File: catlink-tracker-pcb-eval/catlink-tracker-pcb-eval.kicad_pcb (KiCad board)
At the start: 4 copper layers, 36.4 x 38.8 mm, 42 parts, among them J1 S2B-PH-K, J2 U.FL, J3 Header_01x03, J4 Header_02x02, J5 Header_02x03, J6 Header_01x02, J7 Header_01x06, J8 Header_01x05, SW1 SW_Push, U1 STM32L412K8Tx, U2 TLV75530PDBV, U3 Ai-Thinker-Ra-01S, U4 E108-GN03

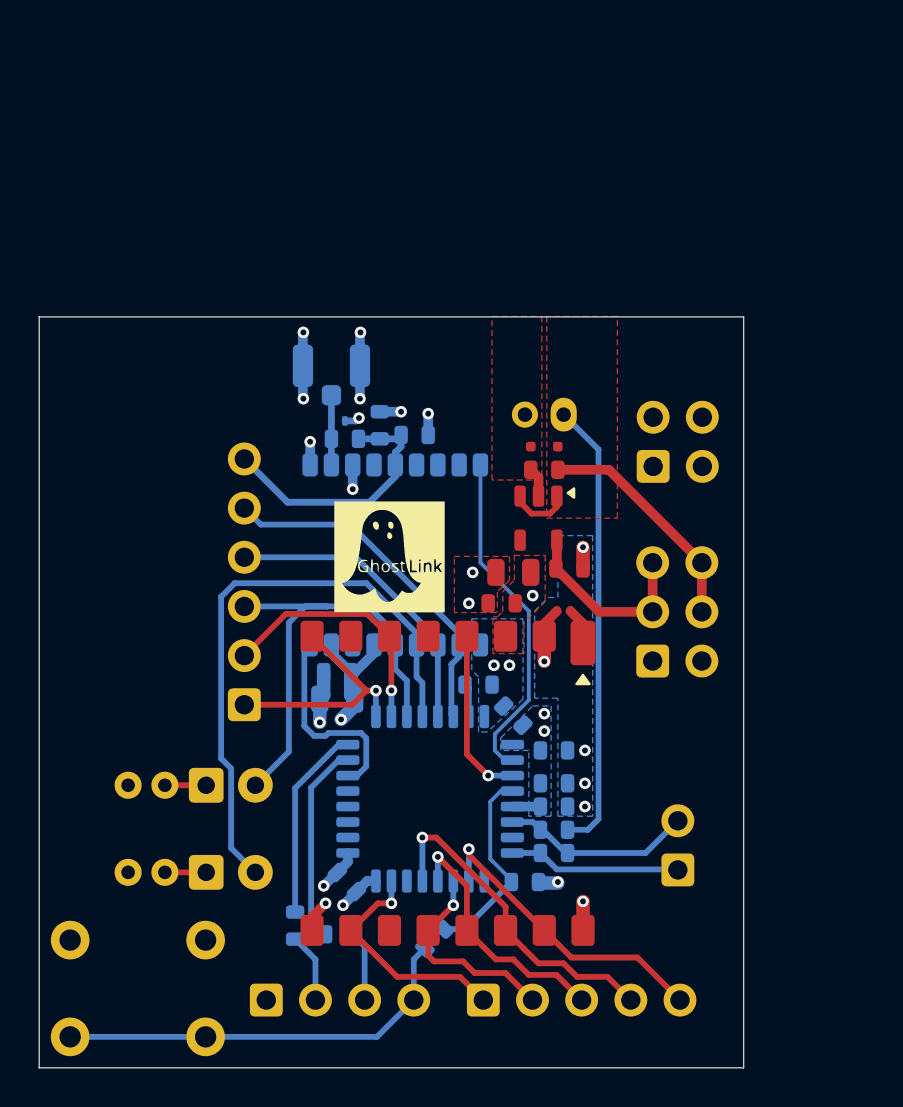
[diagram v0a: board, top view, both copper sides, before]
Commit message: v0.1
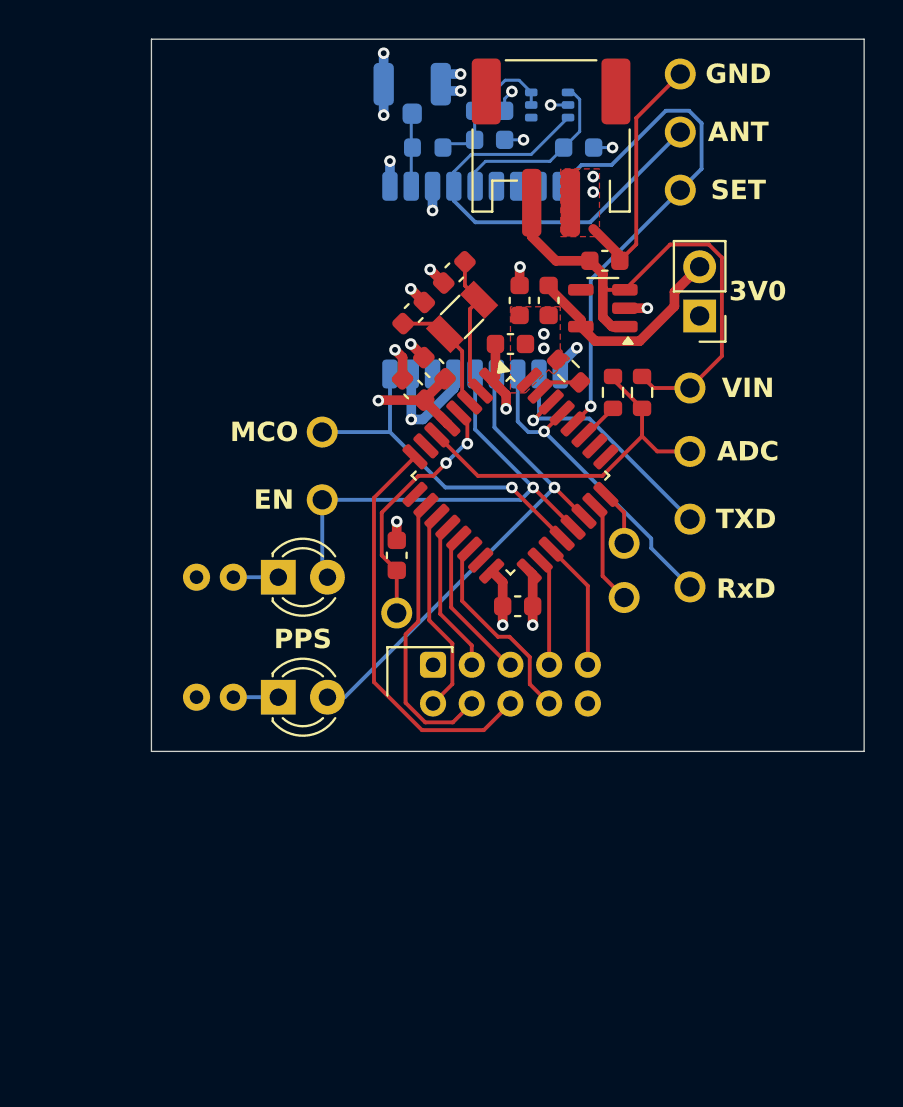
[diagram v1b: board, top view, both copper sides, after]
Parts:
- removed C14: 100p, Custom:C_0603_1608Metric
- removed D2, D3: TPD1E0B04DPY, Custom:D_Texas_DPY0002A_0.6x1mm_P0.65mm
- removed D4: BLUE, LED_THT:LED_D3.0mm
- removed D5: RED, LED_THT:LED_D3.0mm
- removed J4: Header_02x02, Connector_PinHeader_2.54mm:PinHeader_2x02_P2.54mm_Vertical
- removed J5: Header_02x03, Connector_PinHeader_2.54mm:PinHeader_2x03_P2.54mm_Vertical
- removed J6: Header_01x02, Connector_PinHeader_2.54mm:PinHeader_1x02_P2.54mm_Vertical
- removed J7: Header_01x06, Connector_PinHeader_2.54mm:PinHeader_1x06_P2.54mm_Vertical
- removed J8: Header_01x05, Connector_PinHeader_2.54mm:PinHeader_1x05_P2.54mm_Vertical
- removed R6: 100r, Custom:R_0603_1608Metric
- removed R7, R8: 2k, Resistor_THT:R_Axial_DIN0204_L3.6mm_D1.6mm_P1.90mm_Vertical
- removed SW1: SW_Push, Custom:SW_PUSH_5x7mm
- added 3V0: Jumper, Connector_PinHeader_2.54mm:PinHeader_1x02_P2.54mm_Vertical, F.Cu at (135.6, 92.0)
- added ADC: ~, Custom:TestPoint, F.Cu at (135.1, 99.0)
- added ANT: ~, Custom:TestPoint, F.Cu at (134.6, 82.5)
- added EN: ~, Custom:TestPoint, F.Cu at (116.1, 101.5)
- added GND: ~, Custom:TestPoint, F.Cu at (134.6, 79.5)
- added MCO: ~, Custom:TestPoint, F.Cu at (116.1, 98.0)
- added PPS: LED, LED_THT:LED_D3.0mm, F.Cu at (113.9, 111.8)
- added RxD: ~, Custom:TestPoint, F.Cu at (135.1, 106.0)
- added SET: ~, Custom:TestPoint, F.Cu at (134.6, 85.5)
- added TP1: ~, Custom:TestPoint, F.Cu at (120.0, 107.4)
- added TP2: ~, Custom:TestPoint, F.Cu at (131.7, 106.6)
- added TP3: ~, Custom:TestPoint, F.Cu at (131.7, 103.8)
- added TXD: ~, Custom:TestPoint, F.Cu at (135.1, 102.5)
- added VIN: ~, Custom:TestPoint, F.Cu at (135.1, 95.8)
- added Y1: ABS07-32.768KHZ, Crystal:Crystal_SMD_3215-2Pin_3.2x1.5mm, F.Cu at (123.3, 92.1)
- C1, C2, C3, C4, C5, C6: footprint Custom:C_0603_1608Metric -> Capacitor_SMD:C_0603_1608Metric; moved to F.Cu
- C10, C12: value 100n -> 1u; footprint Custom:C_0603_1608Metric -> Capacitor_SMD:C_0603_1608Metric
- C11, C9: value 10u -> 1u; footprint Custom:C_0805_2012Metric -> Capacitor_SMD:C_0603_1608Metric
- C13: value 100n -> 10n; footprint Custom:C_0603_1608Metric -> Capacitor_SMD:C_0603_1608Metric
- C7, C8: value 1u -> 18p; footprint Custom:C_0603_1608Metric -> Capacitor_SMD:C_0603_1608Metric
- D1: value ESD5Z6.0T1G -> LED; footprint Custom:D_SOD-523 -> LED_THT:LED_D3.0mm
- G***: moved to B.Cu
- J1: value S2B-PH-K -> S2B-PH-SM4; footprint Connector_JST:JST_PH_S2B-PH-K_1x02_P2.00mm_Horizontal -> Connector_JST:JST_PH_S2B-PH-SM4-TB_1x02-1MP_P2.00mm_Horizontal; moved to F.Cu
- J2: value U.FL -> S10B-PHDSS; footprint Connector_Coaxial:U.FL_Hirose_U.FL-R-SMT-1_Vertical -> Connector_JST:JST_PHD_S10B-PHDSS_2x05_P2.00mm_Horizontal; moved to F.Cu
- J3: value Header_01x03 -> U.FL; footprint Connector_PinHeader_2.54mm:PinHeader_1x04_P2.54mm_Vertical -> Connector_Coaxial:U.FL_Hirose_U.FL-R-SMT-1_Vertical
- L1: value 82n -> 68nH; footprint Custom:L_0603_1608Metric -> Inductor_SMD:L_0603_1608Metric
- R1, R2, R3: footprint Custom:R_0603_1608Metric -> Resistor_SMD:R_0603_1608Metric; moved to F.Cu
- R4: value 10k -> R; footprint Custom:R_0603_1608Metric -> Resistor_THT:R_Axial_DIN0204_L3.6mm_D1.6mm_P1.90mm_Vertical; moved to F.Cu
- R5: value 100r -> R; footprint Custom:R_0603_1608Metric -> Resistor_THT:R_Axial_DIN0204_L3.6mm_D1.6mm_P1.90mm_Vertical; moved to F.Cu
- U1: footprint Custom:LQFP-32_7x7mm_P0.8mm -> Package_QFP:LQFP-32_7x7mm_P0.8mm; moved to F.Cu
- U2: footprint Custom:SOT-23-5 -> Package_TO_SOT_SMD:SOT-23-5
- U3: value Ai-Thinker-Ra-01S -> E108-GN03; footprint Custom:Ai-Thinker-Ra-01S -> Custom:E108-GN03; moved to B.Cu
- U4: value E108-GN03 -> TPS22919DCKR; footprint Custom:E108-GN03 -> Package_TO_SOT_SMD:SOT-363_SC-70-6
- moved J3 47.5 mm to (120.8, 80.5), turned to 90 degrees
- moved C11 31.1 mm to (129.4, 83.3), turned to 0 degrees
- moved C12 30.1 mm to (124.8, 81.5), turned to 0 degrees
- moved U3 26.0 mm to (124.0, 90.2), turned to 90 degrees
- moved U4 24.6 mm to (127.9, 81.2), turned to 180 degrees
- moved R3 24.0 mm to (131.2, 96.0), turned to 90 degrees
- moved C1 23.3 mm to (126.3, 91.2), turned to -90 degrees
- moved R2 23.1 mm to (132.7, 96.0), turned to 90 degrees
- moved C4 22.7 mm to (120.8, 95.8), turned to 135 degrees
- moved C5 22.3 mm to (121.9, 94.8), turned to 135 degrees
- moved R4 21.4 mm to (111.5, 105.5), turned to 180 degrees
- moved C2 19.2 mm to (125.8, 93.5), turned to 0 degrees
- moved C6 18.1 mm to (120.0, 104.4), turned to -90 degrees
- moved U1 17.2 mm to (125.8, 100.3), turned to -45 degrees
- moved R1 16.9 mm to (128.8, 94.9), turned to -45 degrees
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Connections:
- C1 pad 1: +3V0 -> +3.0V
- C10 pad 1: +3V0 -> Net-(J4-Pin_2)
- C11 pad 1: +3V0 -> /GNSS_VCC_RF
- C12 pad 1: +3V0 -> Net-(U4-QOD)
- C13 pad 1: /VCC_RF -> Net-(U4-QOD)
- C2 pad 1: +3V0 -> +3.0V
- C3 pad 1: +3V0 -> +3.0V
- C4 pad 1: +3V0 -> +3.0V
- C5 pad 1: +3V0 -> +3.0V
- C6 pad 1: Net-(U1-NRST) -> GND
- C6 pad 2: GND -> /NRST
- C7 pad 1: /VIN -> GND
- C7 pad 2: GND -> /OSC32_IN
- C8 pad 1: /VOUT -> GND
- C8 pad 2: GND -> /OSC32_OUT
- C9 pad 1: +3V0 -> /V_{IN}
- D1 pad 1: /VIN -> Net-(D1-K)
- D1 pad 2: GND -> /GNSS_ON_OFF
- J1 pad 2: /VIN -> /V_{IN}
- J2 pad 1: /RF_IN -> GND
- J2 pad 2: GND -> /SX126x_SCK
- J3 pad 1: GND -> /GNSS_RF_IN
- J3 pad 2: /SWCLK -> GND
- L1 pad 1: /RF_IN -> /GNSS_RF_IN
- L1 pad 2: /VCC_RF -> Net-(U4-QOD)
- R1 pad 1: /BOOT0 -> GND
- R1 pad 2: GND -> /BOOT0
- R2 pad 1: /VIN -> /VIN_ADC
- R2 pad 2: /VIN_ADC -> /V_{IN}
- R3 pad 1: /VIN_ADC -> /VIN_ADC_DIV_EN
- R3 pad 2: /VIN_ADC_DIV_EN -> /VIN_ADC
- R4 pad 1: /~{NRST} -> Net-(D1-K)
- R4 pad 2: Net-(U1-NRST) -> GND
- R5 pad 1: Net-(U1-PA13) -> Net-(D2-K)
- R5 pad 2: /SWDIO -> GND
- U1 pad 1: +3V0 -> +3.0V
- U1 pad 10: /~{NSS} -> /SX126x_BUSY
- U1 pad 11: /SCK -> /SX126x_SCK
- U1 pad 12: /MISO -> /SX126x_MISO
- U1 pad 13: /MOSI -> /SX126x_MOSI
- U1 pad 14: unconnected-(U1-PB0-Pad14) -> /SX126x_NSS
- U1 pad 15: /BUSY -> unconnected-(U1-PB1-Pad15)
- U1 pad 17: +3V0 -> +3.0V
- U1 pad 18: unconnected-(U1-PA8-Pad18) -> /SX126x_REST
- U1 pad 19: unconnected-(U1-PA9-Pad19) -> /SX126x_DIO3
- U1 pad 2: /MODEL_SET -> /OSC32_IN
- U1 pad 20: unconnected-(U1-PA10-Pad20) -> /GNSS_RESET_N
- U1 pad 21: unconnected-(U1-PA11-Pad21) -> /GNSS_ON_OFF
- U1 pad 22: /GNSS_~{NRST} -> /GNSS_1PPS
- U1 pad 23: Net-(U1-PA13) -> /SWDIO
- U1 pad 24: Net-(U1-PA14) -> /SWCLK
- U1 pad 25: /DIO3 -> unconnected-(U1-PA15-Pad25)
- U1 pad 26: /DIO1 -> unconnected-(U1-PB3-Pad26)
- U1 pad 27: /ON_OFF -> /VIN_ADC_DIV_EN
- U1 pad 28: /1PPS -> /GNSS_MODEL_SET
- U1 pad 3: /LoRa_~{NRST} -> /OSC32_OUT
- U1 pad 4: Net-(U1-NRST) -> /NRST
- U1 pad 5: +3V0 -> +3.0V
- U1 pad 8: /VIN_ADC_DIV_EN -> /SX126x_DIO1
- U2 pad 1: /VIN -> /V_{IN}
- U2 pad 3: /VIN -> /V_{IN}
- U2 pad 5: /VOUT -> Net-(J4-Pin_2)
- U3 pad 1: /LoRa_ANT -> GND
- U3 pad 10: /BUSY -> GND
- U3 pad 11: unconnected-(U3-RXEN-Pad11) -> /GNSS_RF_IN
- U3 pad 12: /SCK -> GND
- U3 pad 13: /MISO -> /GNSS_ANT_ON
- U3 pad 14: /MOSI -> /GNSS_VCC_RF
- U3 pad 15: /~{NSS} -> unconnected-(U3-NC-Pad15)
- U3 pad 16: GND -> unconnected-(U3-NC-Pad16)
- U3 pad 2: GND -> /GNSS_TXD
- U3 pad 3: +3V0 -> /GNSS_RxD
- U3 pad 4: /LoRa_~{NRST} -> /GNSS_1PPS
- U3 pad 5: unconnected-(U3-TXEN-Pad5) -> /GNSS_ON_OFF
- U3 pad 6: /DIO1 -> +3.0V
- U3 pad 8: /DIO3 -> +3.0V
- U3 pad 9: GND -> /GNSS_RESET_N
- U4 pad 1: GND -> /GNSS_VCC_RF
- U4 pad 2: /GNSS_TXD -> GND
- U4 pad 3: /GNSS_RxD -> /GNSS_ANT_ON
- U4 pad 4: /1PPS -> unconnected-(U4-NC-Pad4)
- U4 pad 5: /ON_OFF -> Net-(U4-QOD)
- U4 pad 6: +3V0 -> Net-(U4-QOD)
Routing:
- net /VIN: track 38.6 -> 0.00 mm
- net /1PPS: track 30.9 -> 0.00 mm
- net /GNSS_MODEL_SET: track 0.00 -> 27.5 mm, vias 0 -> 1
- net /V_{IN}: track 0.00 -> 27.4 mm
- net /GNSS_1PPS: track 0.00 -> 25.6 mm, vias 0 -> 1
- net /GNSS_ON_OFF: track 0.00 -> 25.3 mm, vias 0 -> 1
- net /ON_OFF: track 24.4 -> 0.00 mm
- net /GNSS_ANT_ON: track 0.00 -> 22.6 mm
- net /~{NRST}: track 21.5 -> 0.00 mm
- net /SX126x_DIO1: track 0.00 -> 21.2 mm
- net +3.0V: track 0.00 -> 19.2 mm, vias 0 -> 5
- net /GNSS_RESET_N: track 0.00 -> 17.7 mm, vias 0 -> 1
- net /MODEL_SET: track 17.6 -> 0.00 mm
- net /MOSI: track 17.2 -> 0.00 mm, vias 1 -> 0
- net /~{NSS}: track 16.0 -> 0.00 mm, vias 1 -> 0
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- added copper zone on In1.Cu, net +3.0V
- removed copper zone on B.Cu, net +3V0
- removed copper zone on F.Cu, net +3V0
- removed copper zone on In1.Cu, net +3V0
- removed copper zone on F.Cu, net /VIN
- removed copper zone on B.Cu, net GND
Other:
- board size 36.4 x 38.8 mm -> 36.8 x 36.8 mm
- board text removed: "3-5.5V"
- board text removed: "ADC"
- board text removed: "BU"
- board text removed: "CK"
- board text removed: "DIO1"
- board text removed: "DIO3"
- board text removed: "DIV_EN"
- board text removed: "EN"
- board text removed: "GND"
- board text removed: "IN|OU"
- board text removed: "IO"
- board text removed: "MI"
- board text removed: "MO"
- board text removed: "NRST"
- board text removed: "NS"
- board text removed: "RxD"
- board text removed: "SC"
- board text removed: "TXD"
- board text removed: "VCCRF"
- board text removed: "|3V"
